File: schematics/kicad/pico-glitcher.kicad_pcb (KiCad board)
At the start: 2 copper layers, 89.8 x 58.4 mm, 72 parts, among them Q1 IRLML2502, Q2 IRF7807PBF, Q3 TPS 79318, Q4 TPS2041, U1 NH245, U2 NH245, X1 BU-SMA-V, X2 BU-SMA, X3 M08X2

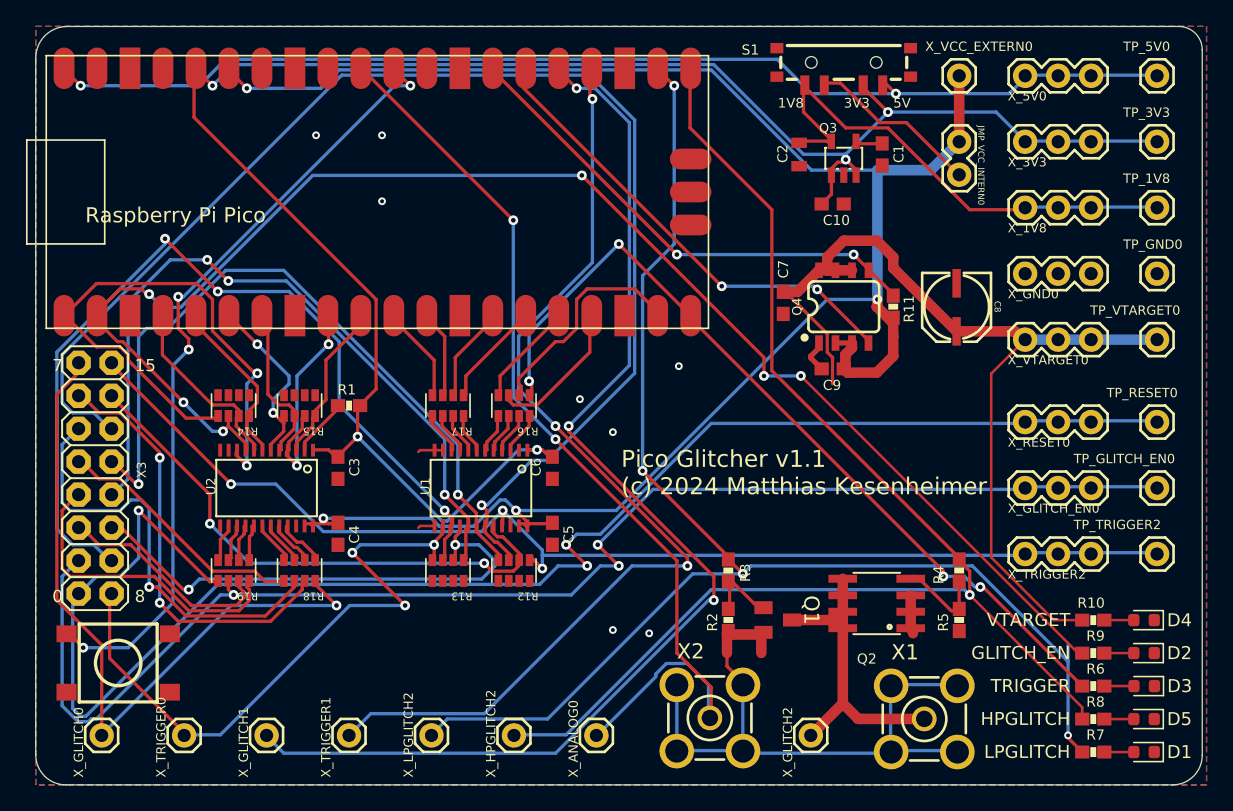
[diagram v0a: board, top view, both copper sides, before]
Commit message: replaced 0603 resistor's symbol and footprint with kicad library's ones
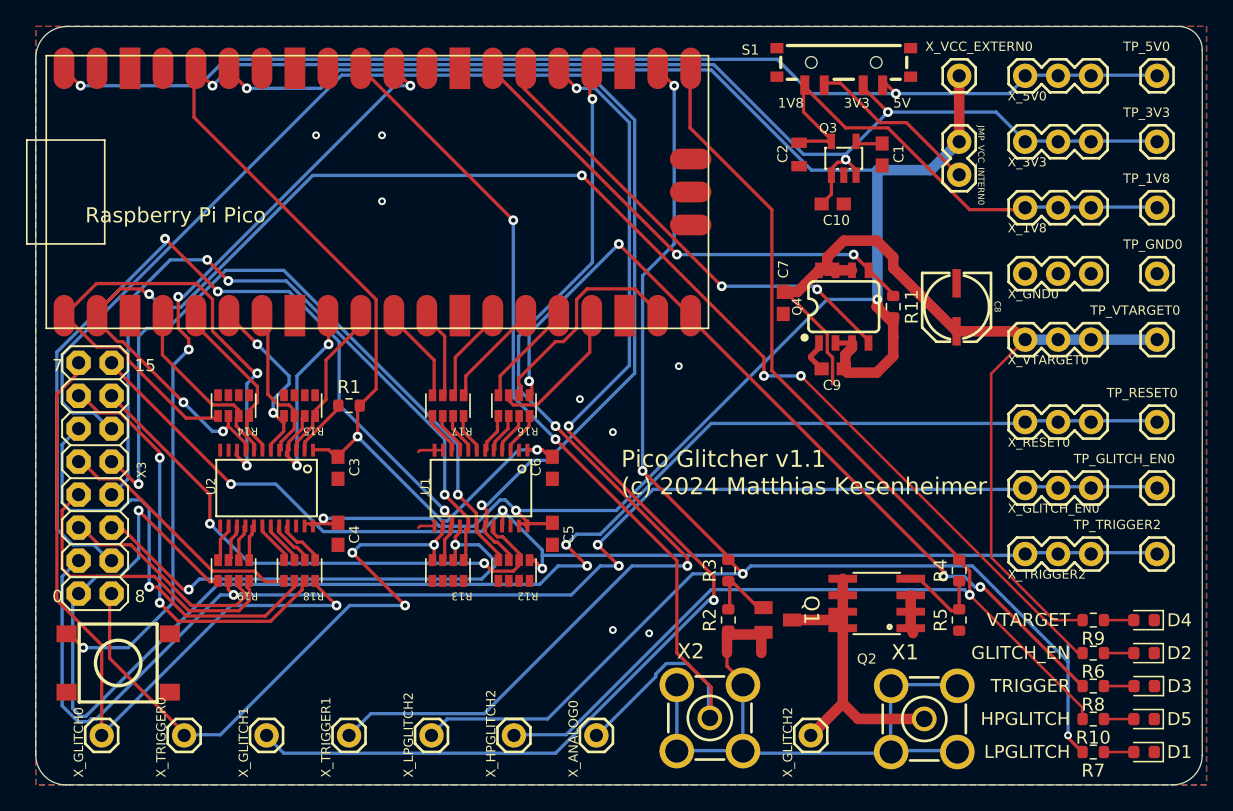
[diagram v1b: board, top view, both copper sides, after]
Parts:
- R1, R10, R11, R2, R3, R4, R5, R6, R7, R8, R9: footprint pico-glitcher:0603-RES -> Resistor_SMD:R_0603_1608Metric
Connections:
- R10 pad 1: Net-(D5-A) -> /HPGLITCH2
- R10 pad 2: /HPGLITCH2 -> Net-(D5-A)
- R2 pad 1: GND -> Net-(Q1-G)
- R2 pad 2: Net-(Q1-G) -> GND
- R4 pad 1: Net-(Q2-G) -> unconnected-(R4-Pad1)
- R4 pad 2: /HPGLITCH2 -> Net-(Q2-G)
- R6 pad 1: Net-(D2-A) -> /GP1
- R6 pad 2: /GP1 -> Net-(D2-A)
- R7 pad 1: Net-(D1-A) -> /LPGLITCH2
- R7 pad 2: /LPGLITCH2 -> Net-(D1-A)
- R8 pad 1: Net-(D3-A) -> /GP15
- R8 pad 2: /GP15 -> Net-(D3-A)
- R9 pad 1: Net-(D4-A) -> /VTARGET
- R9 pad 2: /VTARGET -> Net-(D4-A)
